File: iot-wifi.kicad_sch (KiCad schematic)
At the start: 23 parts, among them J1 USB_C_Receptacle_USB2.0, Q1 DTC114E, Q2 DTC114E, SW1 SW_Push, U1 CP2102N-Axx-xQFN28, U2 ESP32-PICO-D4

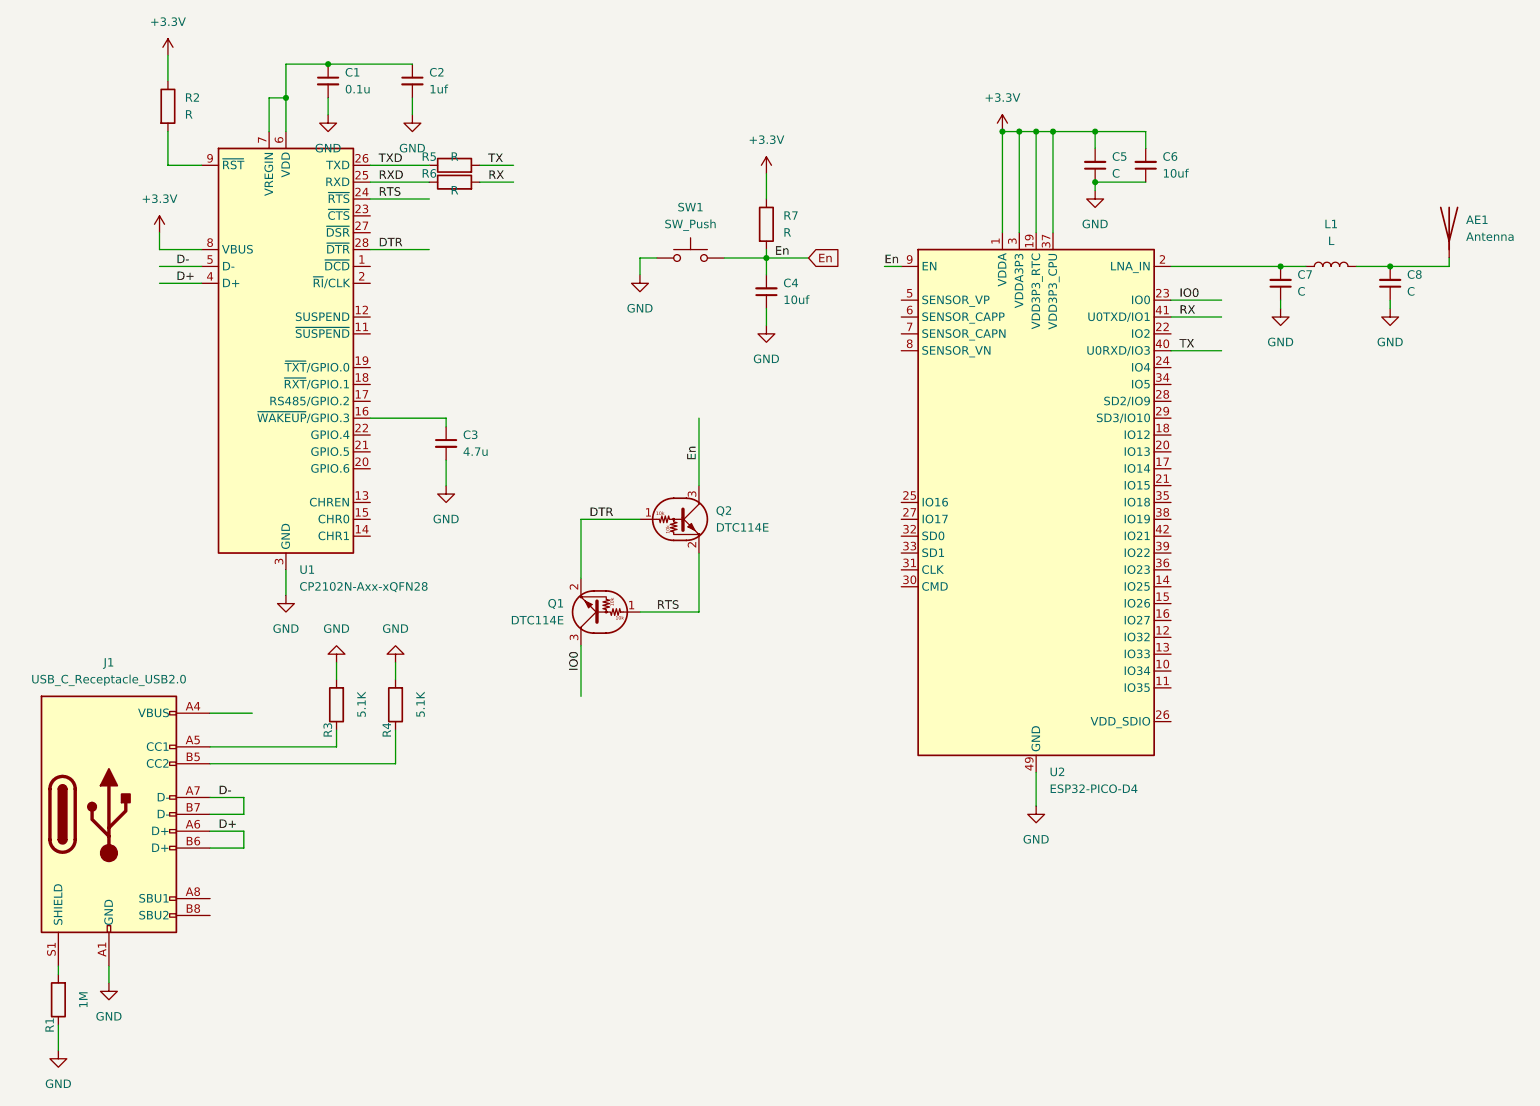
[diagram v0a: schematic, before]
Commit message: ADD: esp32
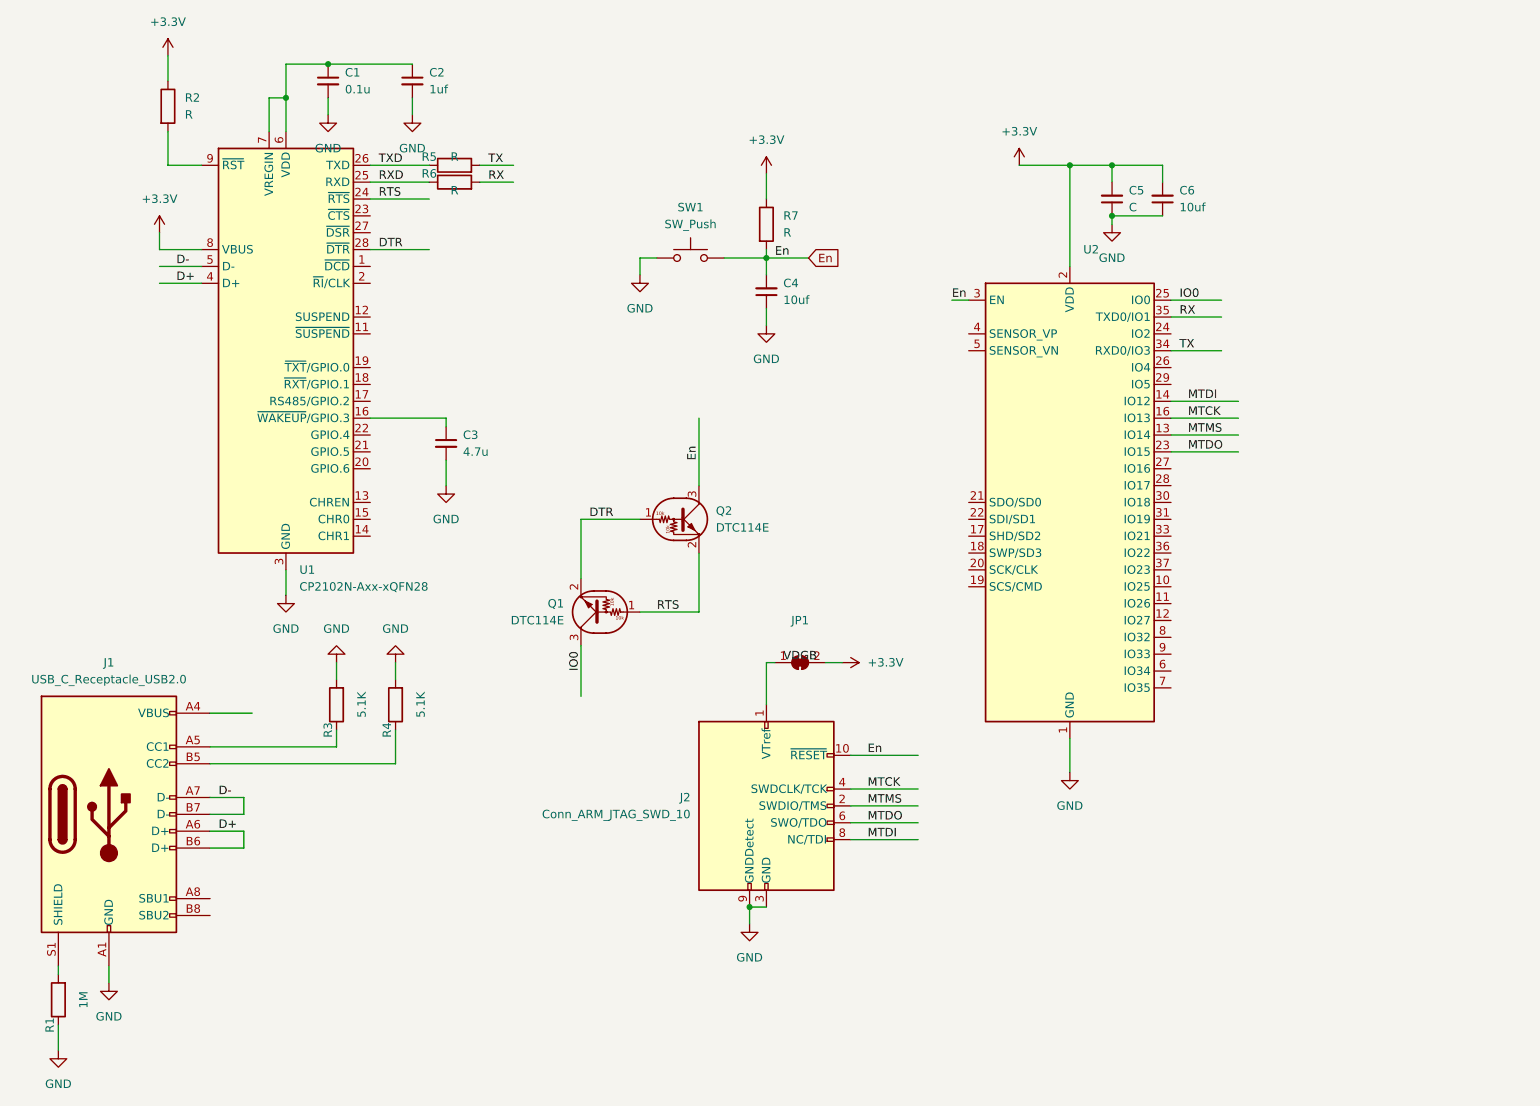
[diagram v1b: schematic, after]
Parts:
- removed AE1: Antenna, symbol Device:Antenna
- removed C7, C8: C, Capacitor_SMD:C_0402_1005Metric_Pad0.74x0.62mm_HandSolder, symbol Device:C_Small
- removed L1: L, Inductor_SMD:L_01005_0402Metric_Pad0.57x0.30mm_HandSolder, symbol Device:L
- removed U2: ESP32-PICO-D4, Package_DFN_QFN:QFN-48-1EP_7x7mm_P0.5mm_EP5.3x5.3mm_ThermalVias, symbol RF_Module:ESP32-PICO-D4
- added J2: Conn_ARM_JTAG_SWD_10, Connector_IDC:IDC-Header_2x05_P2.54mm_Vertical, symbol Connector:Conn_ARM_JTAG_SWD_10
- added JP1: (no value), symbol Jumper:SolderJumper_2_Bridged
- added U2: (no value), symbol RF_Module:ESP32-WROOM-32
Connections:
- net +3V3: now also JP1.2 (B), U2.2 (VDD)
- net En: now also J2.10 (~{RESET}), U2.3 (EN)
- net GND: now also J2.3 (GND), J2.5 (GND), J2.9 (GNDDetect), U2.1 (GND), U2.15 (GND), U2.38 (GND), U2.39 (GND)
- net IO0: now also U2.25 (IO0)
- net RX: now also U2.35 (TXD0/IO1)
- net TX: now also U2.34 (RXD0/IO3)
- new net: J2.1 (VTref), JP1.1 (A)
- new net MTCK: J2.4 (SWDCLK/TCK), U2.16 (IO13)
- new net MTDI: J2.8 (NC/TDI), U2.14 (IO12)
- new net MTDO: J2.6 (SWO/TDO), U2.23 (IO15)
- new net MTMS: J2.2 (SWDIO/TMS), U2.13 (IO14)
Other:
- moved on the sheet: C5, C6
